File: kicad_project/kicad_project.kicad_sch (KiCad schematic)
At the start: 4 parts, among them U1 RP2040

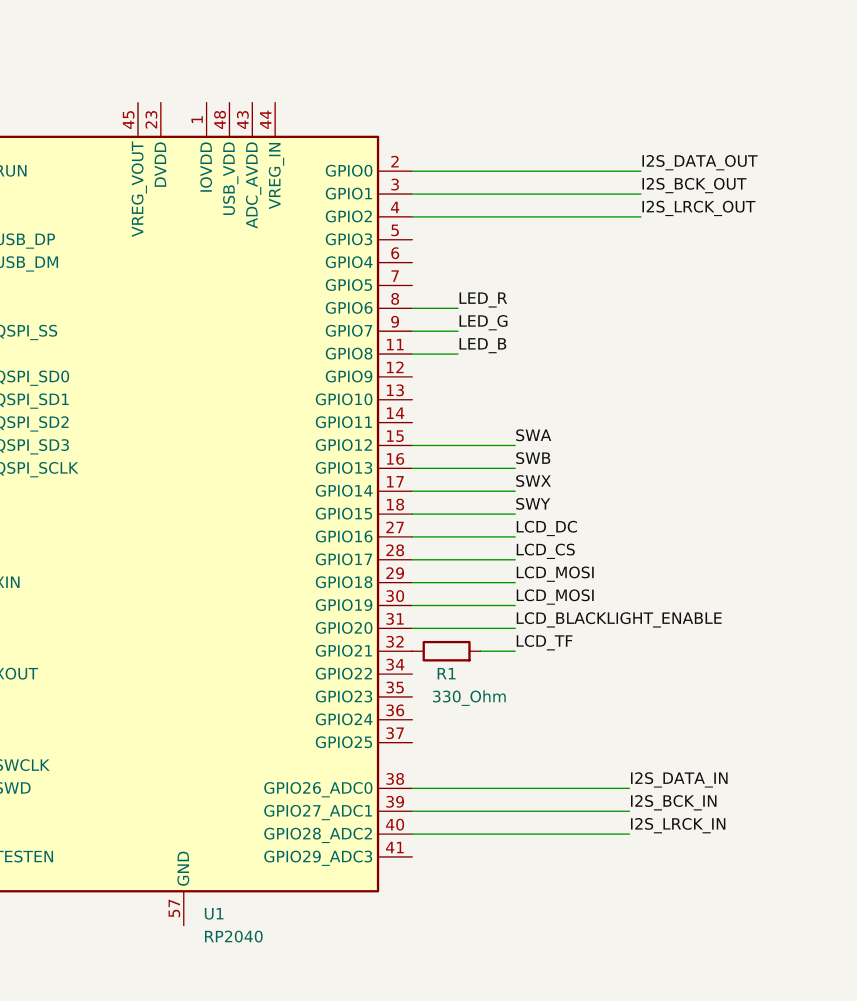
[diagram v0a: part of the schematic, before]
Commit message: Updated KiCAD and played around with the code.
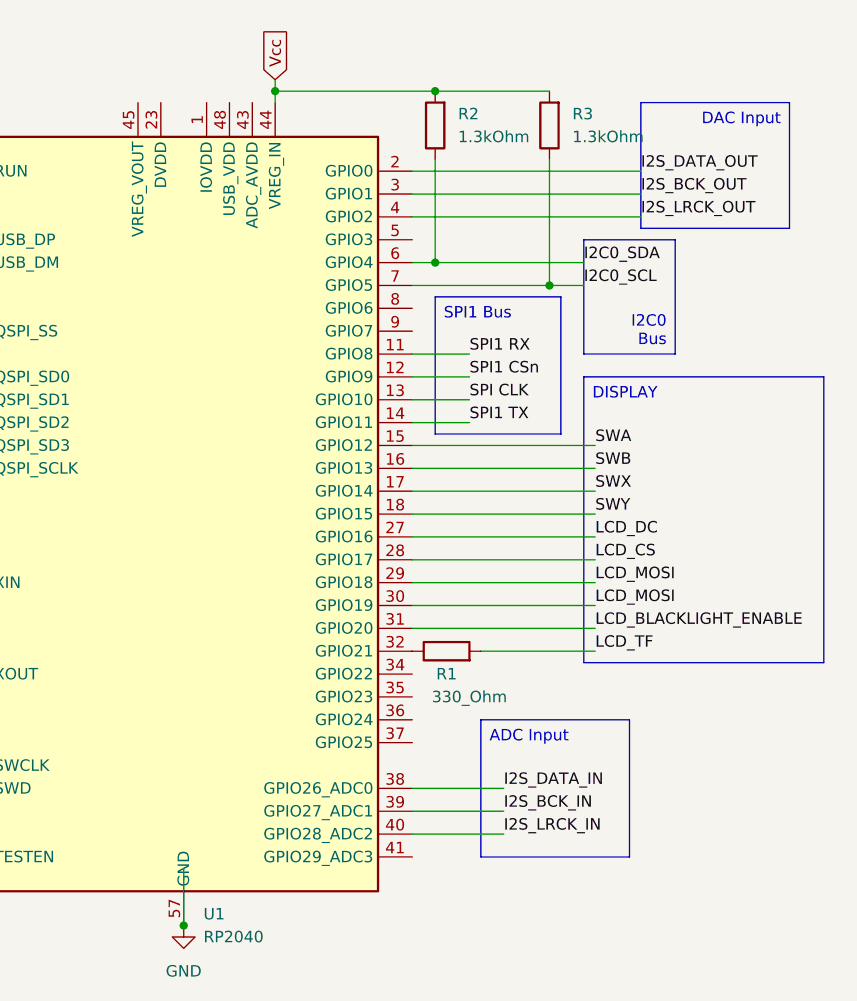
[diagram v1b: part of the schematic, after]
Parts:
- added R2, R3: 1.3kOhm, symbol Device:R
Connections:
- net SPI1 CSn: now reaches U1.12 (GPIO9)
- net SPI CLK: now reaches U1.13 (GPIO10)
- net SPI1 TX: now reaches U1.14 (GPIO11)
- net Vcc: now reaches U1.44 (VREG_IN)
- net Vcc: now also R2.2, R3.2
- net GND: now reaches U1.57 (GND)
- net I2C0_SDA: now reaches U1.6 (GPIO4)
- net I2C0_SDA: now also R2.1
- net I2C0_SCL: now reaches U1.7 (GPIO5)
- net I2C0_SCL: now also R3.1
- net LED_B renamed SPI1 RX
- net LED_G: no longer names the net of U1.9 (GPIO7)
- net LED_R: no longer names the net of U1.8 (GPIO6)
